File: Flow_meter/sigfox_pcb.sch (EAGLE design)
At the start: 15 parts, among them J1 SMA-142-0701-801, U1 SFM11R2D

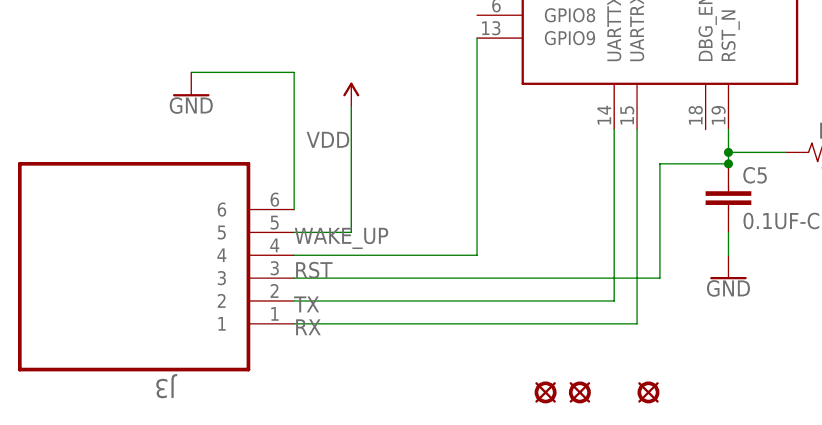
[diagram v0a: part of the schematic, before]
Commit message: First firmware micro Real
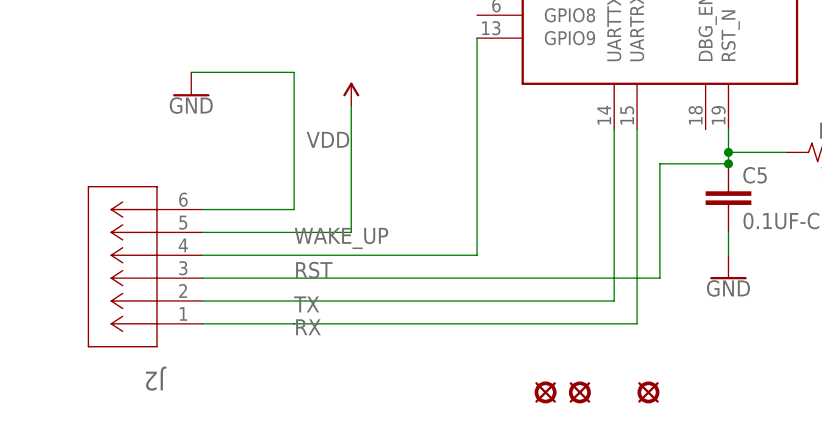
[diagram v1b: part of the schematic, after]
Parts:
- removed J3: (no value), CON_FLUJO:SSW-106-01-T-S
- added J2: SSW-106-02-G-S-RA, SSW-106-02-G_S_RA:SSW-106-02-G-S-RA
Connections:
- net GND: now also J2.6; no longer J3.6
- net RST: now also J2.3; no longer J3.3
- net RX: now also J2.1; no longer J3.1
- net TX: now also J2.2; no longer J3.2
- net VDD: now also J2.5; no longer J3.5
- net WAKE_UP: now also J2.4; no longer J3.4
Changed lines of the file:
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@@
 <part name="H2" library="untitled" deviceset="HOLE" device="-M3"/>
 <part name="H4" library="untitled" deviceset="HOLE" device="-M3"/>
-<part name="J3" library="CON_FLUJO" deviceset="SSW-106-01-T-S" device=""/>
+<part name="J2" library="SSW-106-02-G_S_RA" deviceset="SSW-106-02-G-S-RA" device="" value=""/>
 </parts>
 <sheets>
@@
 <instance part="H2" gate="G$1" x="-8.89" y="-45.72" smashed="yes"/>
 <instance part="H4" gate="G$1" x="-1.27" y="-45.72" smashed="yes"/>
-<instance part="J3" gate="A" x="-53.34" y="-35.56" smashed="yes" rot="R180">
-<attribute name="NAME" x="-53.7718" y="-44.2468" size="2.0828" layer="95" ratio="10" rot="SR180"/>
-<attribute name="VALUE" x="-53.1876" y="-16.9418" size="2.0828" layer="96" ratio="10" rot="SR180"/>
+<instance part="J2" gate="A" x="-50.8" y="-38.1" smashed="yes" rot="R180">
+<attribute name="NAME" x="-54.9656" y="-43.4086" size="2.0828" layer="95" ratio="6" rot="SR180"/>
 </instance>
 </instances>
@@
 </segment>
 <segment>
-<pinref part="J3" gate="A" pin="6"/>
 <wire x1="-40.64" y1="-25.4" x2="-40.64" y2="-10.16" width="0.1524" layer="91"/>
 <pinref part="U$10" gate="G$1" pin="GND"/>
 <wire x1="-40.64" y1="-10.16" x2="-52.07" y2="-10.16" width="0.1524" layer="91"/>
+<pinref part="J2" gate="A" pin="6"/>
+<wire x1="-40.64" y1="-25.4" x2="-50.8" y2="-25.4" width="0.1524" layer="91"/>
 </segment>
 </net>
@@
 <segment>
 <pinref part="U$9" gate="A" pin="VDD"/>
-<pinref part="J3" gate="A" pin="5"/>
 <wire x1="-34.29" y1="-13.97" x2="-34.29" y2="-27.94" width="0.1524" layer="91"/>
-<wire x1="-34.29" y1="-27.94" x2="-40.64" y2="-27.94" width="0.1524" layer="91"/>
+<pinref part="J2" gate="A" pin="5"/>
+<wire x1="-34.29" y1="-27.94" x2="-50.8" y2="-27.94" width="0.1524" layer="91"/>
 </segment>
 </net>
@@
 <pinref part="U1" gate="G$1" pin="RST_N"/>
 <label x="-40.64" y="-33.02" size="1.778" layer="95"/>
-<pinref part="J3" gate="A" pin="3"/>
-<wire x1="-40.64" y1="-33.02" x2="0" y2="-33.02" width="0.1524" layer="91"/>
+<wire x1="-50.8" y1="-33.02" x2="0" y2="-33.02" width="0.1524" layer="91"/>
 <wire x1="0" y1="-33.02" x2="0" y2="-20.32" width="0.1524" layer="91"/>
 <wire x1="0" y1="-20.32" x2="7.62" y2="-20.32" width="0.1524" layer="91"/>
 <junction x="7.62" y="-20.32"/>
+<pinref part="J2" gate="A" pin="3"/>
 </segment>
 </net>
@@
 <label x="-40.64" y="-29.21" size="1.778" layer="95"/>
 <pinref part="U1" gate="G$1" pin="GPIO9"/>
-<pinref part="J3" gate="A" pin="4"/>
-<wire x1="-40.64" y1="-30.48" x2="-20.32" y2="-30.48" width="0.1524" layer="91"/>
+<wire x1="-50.8" y1="-30.48" x2="-20.32" y2="-30.48" width="0.1524" layer="91"/>
 <wire x1="-20.32" y1="-30.48" x2="-20.32" y2="-6.35" width="0.1524" layer="91"/>
+<pinref part="J2" gate="A" pin="4"/>
 </segment>
 </net>
@@
 <label x="-40.64" y="-36.83" size="1.778" layer="95"/>
 <pinref part="U1" gate="G$1" pin="UARTTX"/>
-<pinref part="J3" gate="A" pin="2"/>
 <wire x1="-5.08" y1="-35.56" x2="-5.08" y2="-16.51" width="0.1524" layer="91"/>
-<wire x1="-40.64" y1="-35.56" x2="-5.08" y2="-35.56" width="0.1524" layer="91"/>
+<wire x1="-50.8" y1="-35.56" x2="-5.08" y2="-35.56" width="0.1524" layer="91"/>
+<pinref part="J2" gate="A" pin="2"/>
 </segment>
 </net>
@@
 <label x="-40.64" y="-39.37" size="1.778" layer="95"/>
 <pinref part="U1" gate="G$1" pin="UARTRX"/>
-<pinref part="J3" gate="A" pin="1"/>
-<wire x1="-40.64" y1="-38.1" x2="-2.54" y2="-38.1" width="0.1524" layer="91"/>
-</segment>
-</net>
+<wire x1="-40.64" y1="-38.1" x2="-38.1" y2="-38.1" width="0.1524" layer="91"/>
+<pinref part="J2" gate="A" pin="1"/>
+<wire x1="-38.1" y1="-38.1" x2="-2.54" y2="-38.1" width="0.1524" layer="91"/>
+<wire x1="-50.8" y1="-38.1" x2="-40.64" y2="-38.1" width="0.1524" layer="91"/>
+</segment>
+</net>
